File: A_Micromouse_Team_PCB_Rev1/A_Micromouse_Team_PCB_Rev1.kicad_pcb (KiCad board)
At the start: 2 copper layers, 82 x 129 mm, 23 parts, among them J1 TOF2, J10 5V->12V, J11 MotorCageMount, J12 MotorCageMount, J13 Battery, J2 locked, J3 TOF4, J4 TOF5, J5 Motor1, J6 Motor2, J7 NeoPixel, J8 TOF1, J9 Battery, SW1 SW_DIP_x06, U1 Teensy4.0, U2 IMU, U3 MotorController

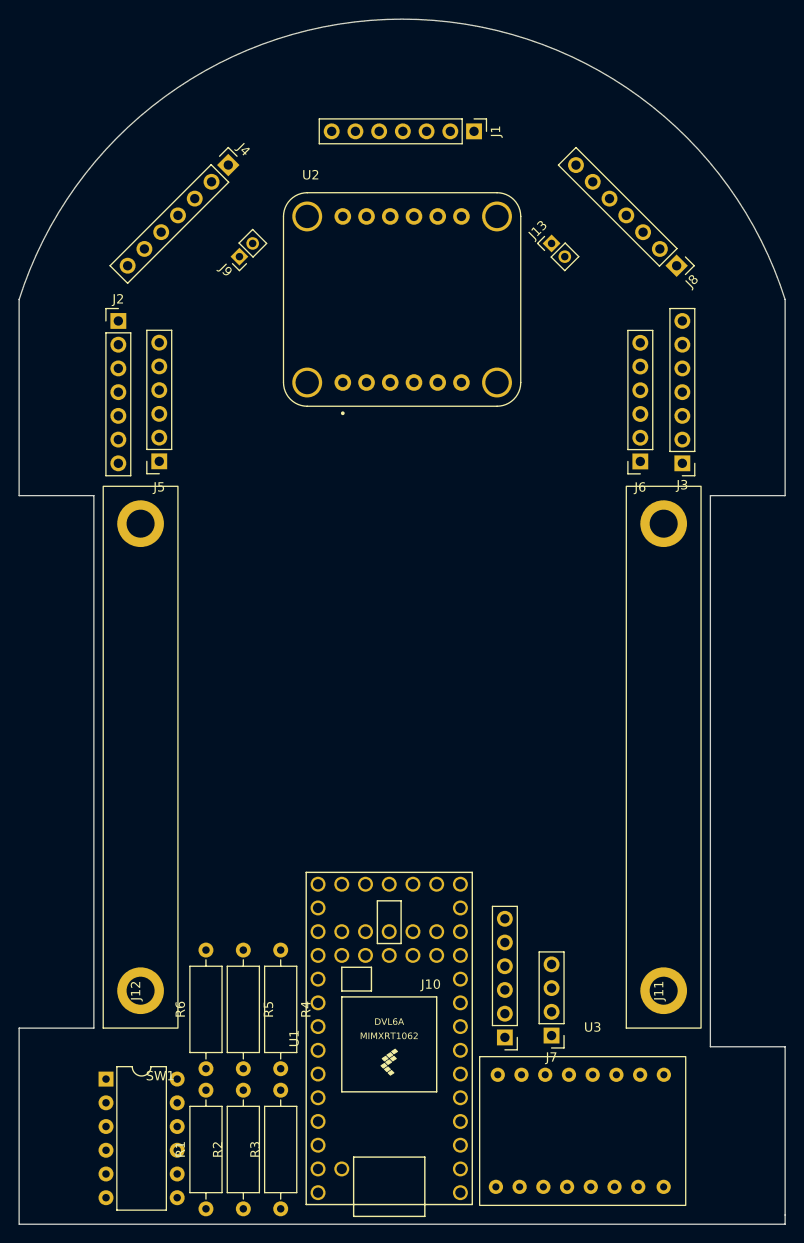
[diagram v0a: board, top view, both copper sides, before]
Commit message: Add files via upload
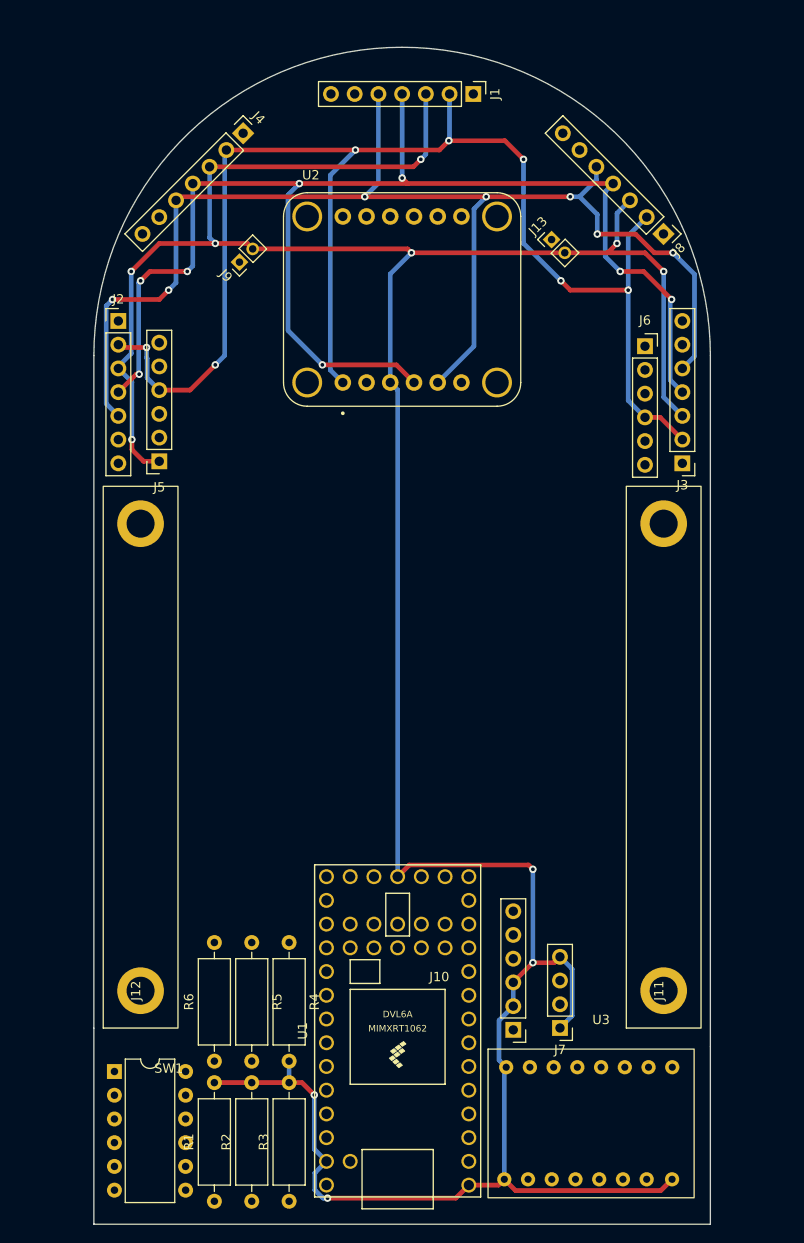
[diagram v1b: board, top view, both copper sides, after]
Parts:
- moved J6 12.4 mm to (171.0, 80.0), turned to 0 degrees
- moved J1 4.00 mm to (152.6, 53.0)
- moved J4 3.76 mm to (128.0, 57.2)
- moved J8 3.69 mm to (173.0, 68.0)
- moved J10 1.21 mm to (156.9, 153.2)
- moved J7 1.21 mm to (161.9, 153.0)
- moved R1 1.21 mm to (124.9, 171.5)
- moved R2 1.21 mm to (128.9, 171.5)
- moved R3 1.21 mm to (132.9, 171.5)
- moved R4 1.21 mm to (132.9, 143.8)
- moved R5 1.21 mm to (128.9, 143.8)
- moved R6 1.21 mm to (124.9, 156.5)
- moved SW1 1.21 mm to (114.2, 157.7)
- moved U1 1.21 mm to (144.5, 153.3)
- moved U3 1.21 mm to (156.1, 157.2)
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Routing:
- net GND: track 0.00 -> 340.1 mm, vias 0 -> 11
- net +5V: track 0.00 -> 153.8 mm, vias 0 -> 7
- net SDA: track 0.00 -> 142.7 mm, vias 0 -> 8
- net SCL: track 0.00 -> 138.2 mm, vias 0 -> 7
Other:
- board size 82 x 129 mm -> 66 x 126 mm
